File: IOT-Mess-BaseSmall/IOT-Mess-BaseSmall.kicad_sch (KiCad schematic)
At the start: 21 parts, among them J1 ESP_P16 / ESP12, J10 Jumper_2, J11 Jumper_2, J12 Jumper_2, J13 Jumper_2, J14 Jumper_2, J15 Jumper_2, J16 Jumper_2, J17 Jumper_2, J18 Jumper_2, J19 Jumper_2, J2 ESP_P16 / C3, J20 Jumper_2, J21 Jumper_2, J3 ESP_P40, J4 Jumper_2, J5 Lolin32-Lite, J6 CH582, J7 Jumper_2, J8 Jumper_2, J9 Jumper_2

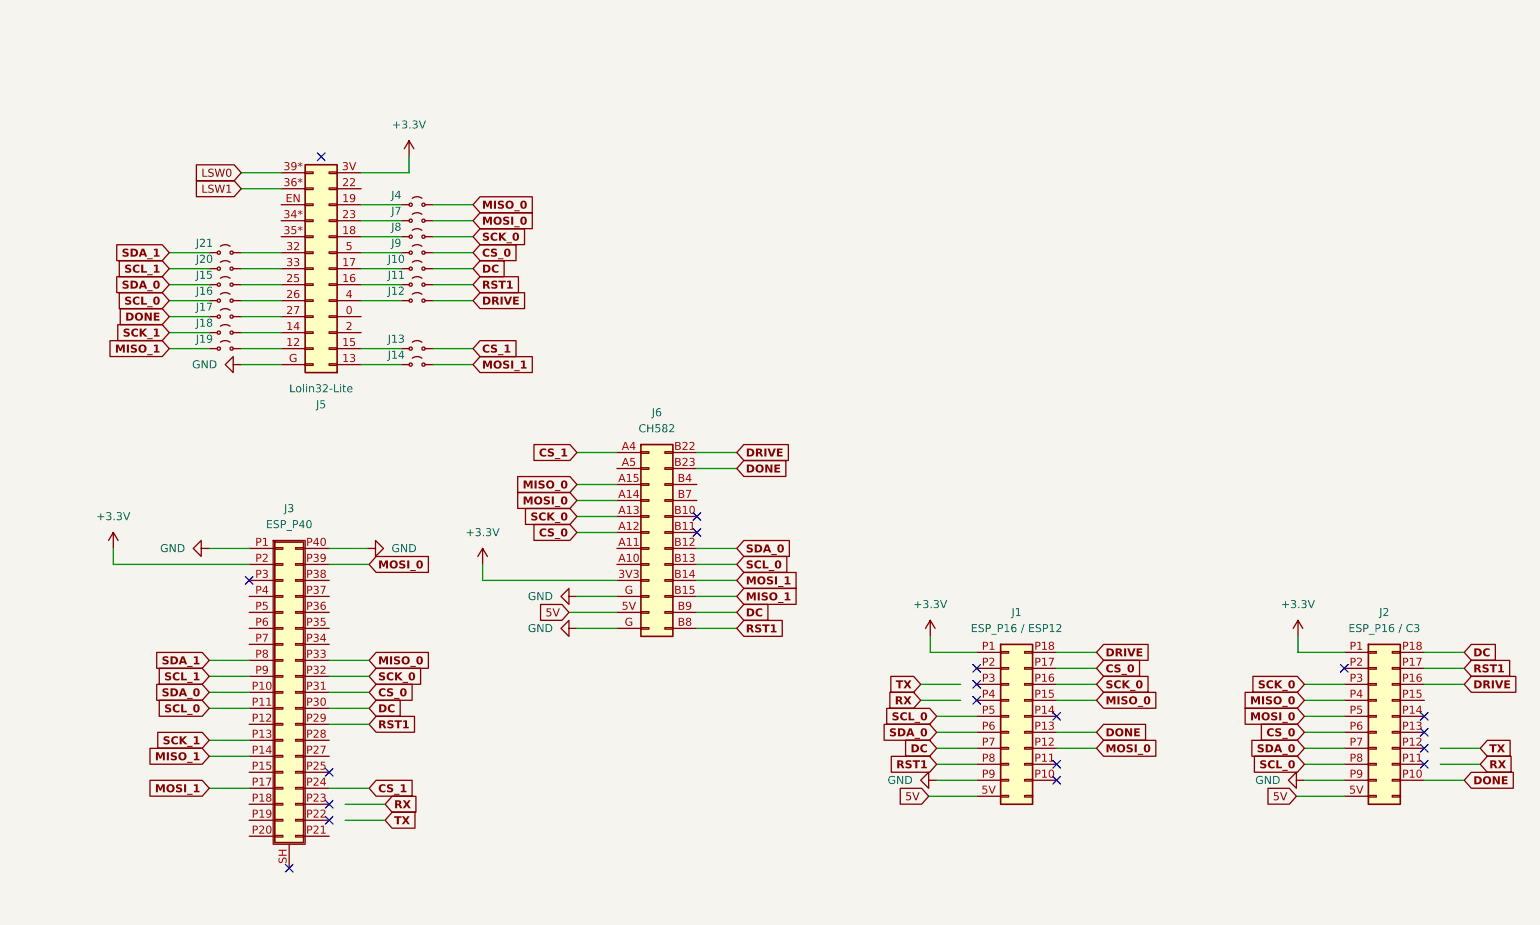
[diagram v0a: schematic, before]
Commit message: did some works.
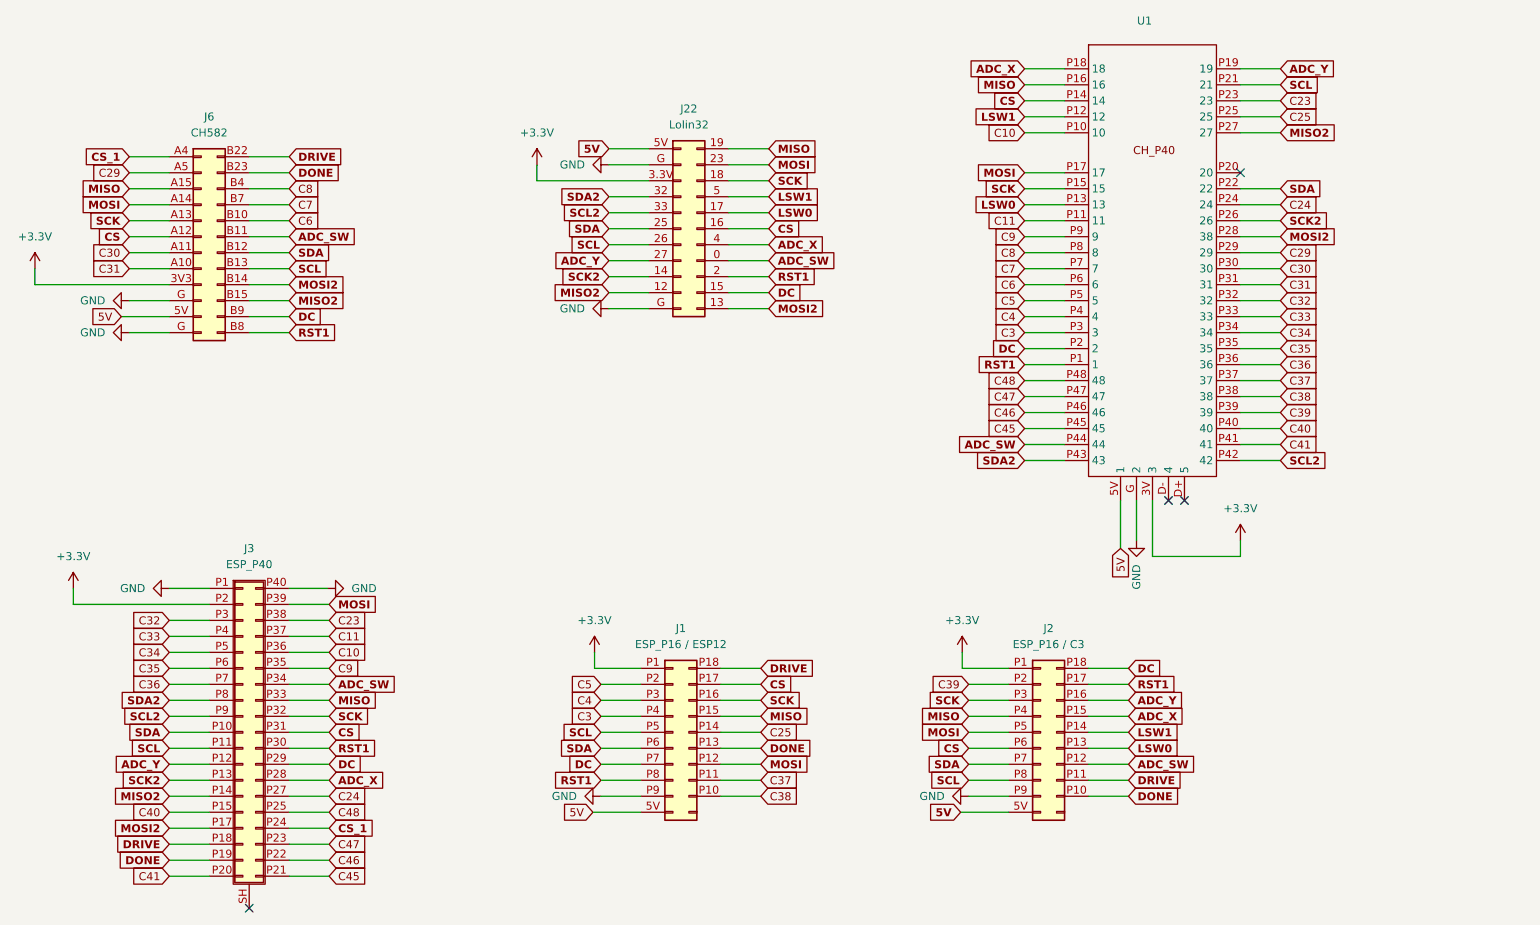
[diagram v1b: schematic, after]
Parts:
- removed J10, J11, J12, J13, J14, J15, J16, J17, J18, J19, J20, J21, J4, J7, J8, J9: Jumper_2, IOT-Mess-Footprints:Jumpper-triangle, symbol Jumper:Jumper_2_Small_Open
- removed J5: Lolin32-Lite, IOT-Mess-Footprints:Lolin32_Lite2, symbol IOT-Mess:Lolin32-Lite
- added J22: Lolin32, IOT-Mess-Footprints:Lolin32-Adapter, symbol Connector_Generic:Conn_02x11_Top_Bottom
- added U1: ~, IOT-Mess-Footprints:CH_P48, symbol IOT-Mess:ESP_P40
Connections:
- net +3.3V: now also J22.3.3V (Pin_3), U1.3V (3)
- net 5V: now also J22.5V (Pin_1), U1.5V (1)
- net DC: now also J3.P29 (Pin_31), J22.15 (Pin_21), U1.P2 (2); no longer J3.P30 (Pin_30)
- net DONE: now also J3.P19 (Pin_18)
- net DRIVE: now also J2.P11 (Pin_13), J3.P18 (Pin_17); no longer J2.P16 (Pin_18)
- net GND: now also J22.G (Pin_11), U1.G (2)
- net LSW0: now also J2.P13 (Pin_15), J22.17 (Pin_16), U1.P13 (13)
- net LSW1: now also J2.P14 (Pin_16), J22.5 (Pin_15), U1.P12 (12)
- net RST1: now also J3.P30 (Pin_30), J22.2 (Pin_20), U1.P1 (1); no longer J3.P29 (Pin_31)
- net C31: now reaches J6.A10 (Pin_8)
- net C31: now also U1.P31 (31)
- net C30: now reaches J6.A11 (Pin_7)
- net C30: now also U1.P30 (30)
- net C29: now reaches J6.A5 (Pin_2)
- net C29: now also U1.P29 (29)
- net C6: now reaches J6.B10 (Pin_17)
- net C6: now also U1.P6 (6)
- net ADC_SW: now reaches J6.B11 (Pin_18)
- net ADC_SW: now also J2.P12 (Pin_14), J3.P34 (Pin_26), J22.0 (Pin_19), U1.P44 (44)
- net C8: now reaches J6.B4 (Pin_15)
- net C8: now also U1.P8 (8)
- net C7: now reaches J6.B7 (Pin_16)
- net C7: now also U1.P7 (7)
- net ADC_Y: now reaches J3.P12 (Pin_12)
- net ADC_Y: now also J2.P16 (Pin_18), J22.27 (Pin_8), U1.P19 (19)
- net C40: now reaches J3.P15 (Pin_15)
- net C40: now also U1.P40 (40)
- net C41: now reaches J3.P20 (Pin_19)
- net C41: now also U1.P41 (41)
- net C45: now reaches J3.P21 (Pin_38)
- net C45: now also U1.P45 (45)
- net C46: now reaches J3.P22 (Pin_37)
- net C46: now also U1.P46 (46)
- net C47: now reaches J3.P23 (Pin_36)
- net C47: now also U1.P47 (47)
- net C48: now reaches J3.P25 (Pin_34)
- net C48: now also U1.P48 (48)
- net C24: now reaches J3.P27 (Pin_33)
- net C24: now also U1.P24 (24)
- net ADC_X: now reaches J3.P28 (Pin_32)
- net ADC_X: now also J2.P15 (Pin_17), J22.4 (Pin_18), U1.P18 (18)
- net C32: now reaches J3.P3 (Pin_3)
- net C32: now also U1.P32 (32)
- net C9: now reaches J3.P35 (Pin_25)
- net C9: now also U1.P9 (9)
- net C10: now reaches J3.P36 (Pin_24)
- net C10: now also U1.P10 (10)
- net C11: now reaches J3.P37 (Pin_23)
- net C11: now also U1.P11 (11)
- net C23: now reaches J3.P38 (Pin_22)
- net C23: now also U1.P23 (23)
- net C33: now reaches J3.P4 (Pin_4)
- net C33: now also U1.P33 (33)
- net C34: now reaches J3.P5 (Pin_5)
- net C34: now also U1.P34 (34)
- net C35: now reaches J3.P6 (Pin_6)
- net C35: now also U1.P35 (35)
- net C36: now reaches J3.P7 (Pin_7)
- net C36: now also U1.P36 (36)
- net C38: now reaches J1.P10 (Pin_12)
- net C38: now also U1.P38 (38)
- net C37: now reaches J1.P11 (Pin_13)
- net C37: now also U1.P37 (37)
- net C25: now reaches J1.P14 (Pin_16)
- net C25: now also U1.P25 (25)
- net C5: now reaches J1.P2 (Pin_2)
- net C5: now also U1.P5 (5)
- net C4: now reaches J1.P3 (Pin_3)
- net C4: now also U1.P4 (4)
- net C3: now reaches J1.P4 (Pin_4)
- net C3: now also U1.P3 (3)
- net C39: now reaches J2.P2 (Pin_2)
- net C39: now also U1.P39 (39)
- net CS_0 renamed CS
- net CS: now also J22.16 (Pin_17), U1.P14 (14)
- net MISO_0 renamed MISO
- net MISO: now also J22.19 (Pin_12), U1.P16 (16)
- net MISO_1 renamed MISO2
- net MISO2: now also J22.12 (Pin_10), U1.P27 (27)
- net MOSI_0 renamed MOSI
- net MOSI: now also J22.23 (Pin_13), U1.P17 (17)
- net MOSI_1 renamed MOSI2
- net MOSI2: now also J22.13 (Pin_22), U1.P28 (38)
- net SCK_0 renamed SCK
- net SCK: now also J22.18 (Pin_14), U1.P15 (15)
- net SCK_1 renamed SCK2
- net SCK2: now also J22.14 (Pin_9), U1.P26 (26)
- net SCL_0 renamed SCL
- net SCL: now also J22.26 (Pin_7), U1.P21 (21)
- net SCL_1 renamed SCL2
- net SCL2: now also J22.33 (Pin_5), U1.P42 (42)
- net SDA_0 renamed SDA
- net SDA: now also J22.25 (Pin_6), U1.P22 (22)
- net SDA_1 renamed SDA2
- net SDA2: now also J22.32 (Pin_4), U1.P43 (43)
- no-connect marks 19 -> 4
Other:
- moved on the sheet: J1, J2, J3, J6
